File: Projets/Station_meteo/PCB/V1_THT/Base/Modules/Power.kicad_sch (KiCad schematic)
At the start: 7 parts, among them U2 AMS1117-3.3

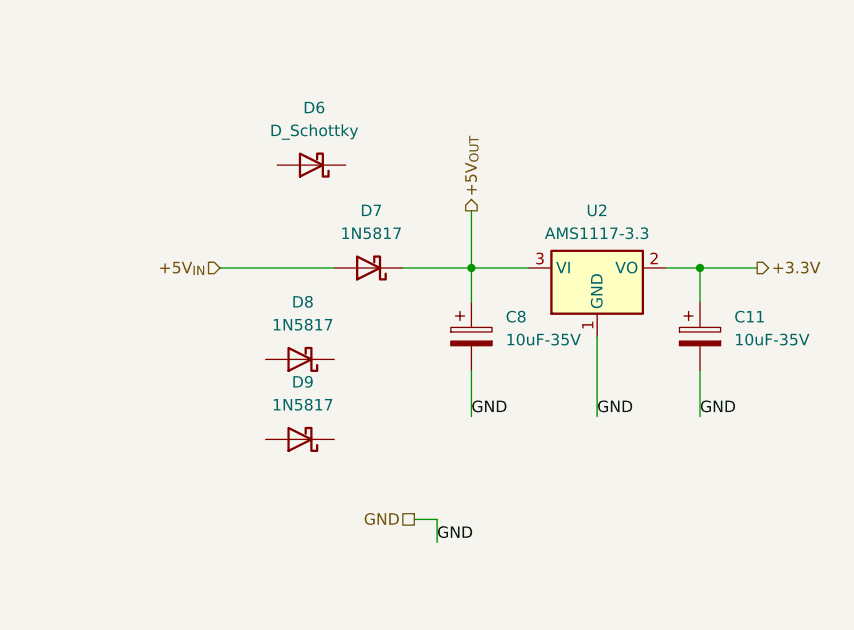
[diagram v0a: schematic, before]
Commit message: Update Schematic
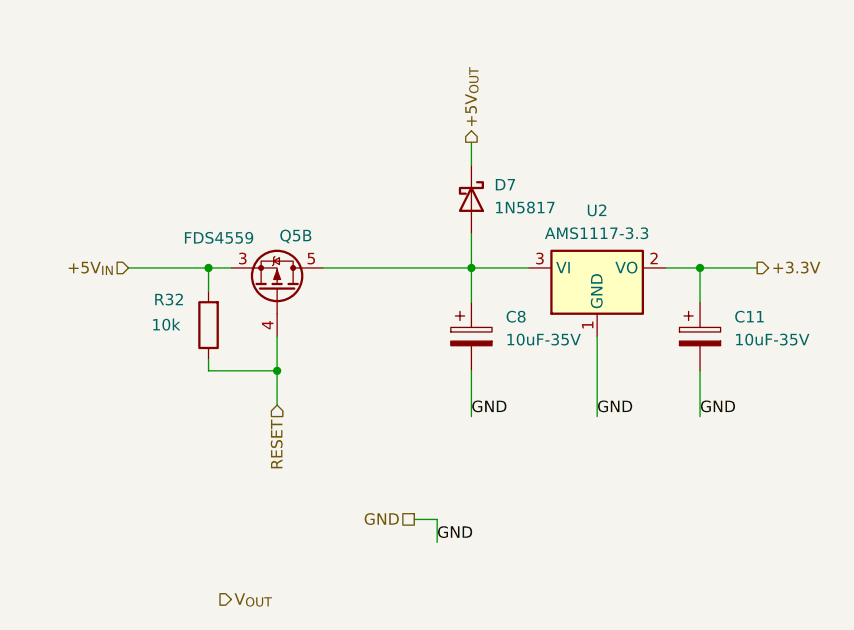
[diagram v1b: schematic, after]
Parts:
- removed D6: D_Schottky, symbol Device:D_Schottky
- removed D8, D9: 1N5817, Diode_THT:D_DO-41_SOD81_P10.16mm_Horizontal, symbol Diode:1N5817
- added Q5: FDS4559, Package_SO:SOIC-8_3.9x4.9mm_P1.27mm, symbol Transistor_FET:FDS4559
- added R32: 10k, Resistor_THT:R_Axial_DIN0207_L6.3mm_D2.5mm_P7.62mm_Horizontal, symbol Device:R
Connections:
- net +5V_{IN}: now also Q5.3 (1), R32.2; no longer D7.2 (A)
- net +5V_{OUT}: no longer C8.1, U2.3 (VI)
- new net: C8.1, D7.2 (A), Q5.5 (D), Q5.6 (D), U2.3 (VI)
- new net RESET: Q5.4 (G), R32.1
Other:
- moved on the sheet: D7
